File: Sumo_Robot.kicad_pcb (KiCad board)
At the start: 4 copper layers, 90 x 90 mm, 65 parts, among them J10 Screw_Terminal_01x03, J12 Screw_Terminal_01x02, J14 Screw_Terminal_01x02, J15 Conn_01x02, J16 Conn_01x03, J17 Conn_01x08, J18 Conn_01x02, J19 Conn_01x02, J2 Screw_Terminal_01x04, J3 Screw_Terminal_01x04, J4 Screw_Terminal_01x04, J5 Screw_Terminal_01x04, J6 Screw_Terminal_01x04, J7 Screw_Terminal_01x03, J8 Screw_Terminal_01x03, J9 Screw_Terminal_01x03, SW1 SW_SPST, SW3 SW_Omron_B3FS, U5 AMS1117-3.3, U6 TSOP38233

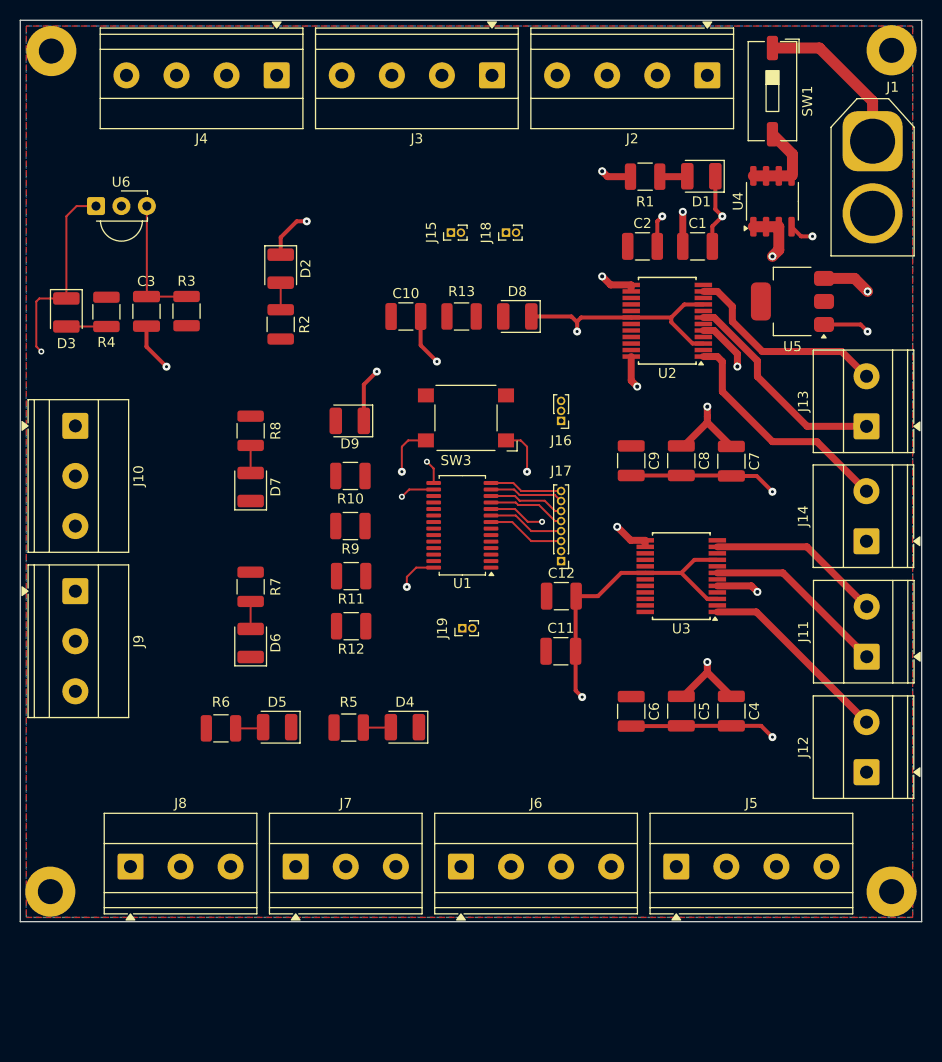
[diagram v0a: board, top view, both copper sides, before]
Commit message: updating layout
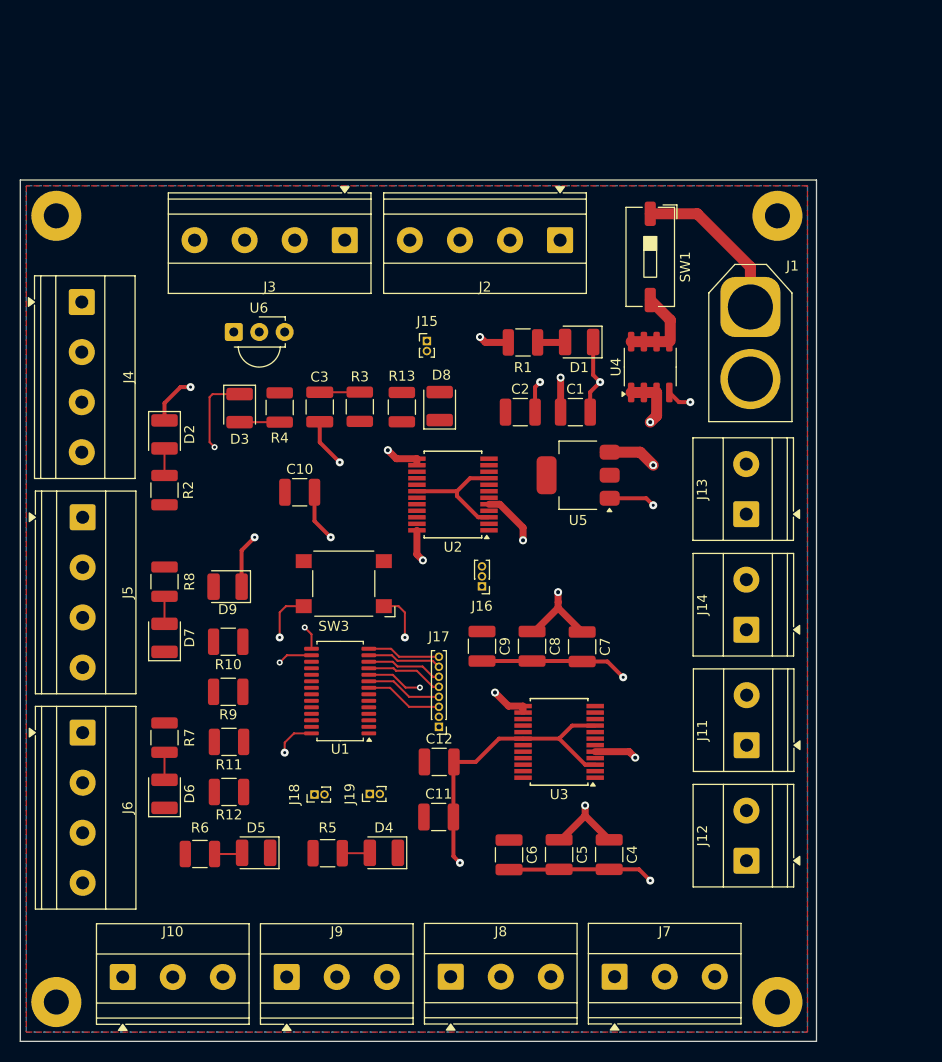
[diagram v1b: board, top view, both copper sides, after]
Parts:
- moved J5 68.8 mm to (110.1, 87.0), turned to -90 degrees
- moved J18 59.3 mm to (133.3, 114.7)
- moved J10 55.2 mm to (114.1, 133.0), turned to 0 degrees
- moved J9 43.9 mm to (130.5, 132.9), turned to 0 degrees
- moved J6 40.1 mm to (110.1, 108.5), turned to -90 degrees
- moved J8 33.8 mm to (146.9, 132.9)
- moved J7 33.7 mm to (163.2, 132.9)
- moved J4 29.8 mm to (110.0, 65.6), turned to -90 degrees
- moved U2 27.5 mm to (147.1, 84.8)
- moved U5 27.5 mm to (159.6, 82.8)
- moved C7 23.8 mm to (160.0, 100.0)
- moved C8 23.8 mm to (155.0, 99.9)
- moved C9 23.8 mm to (150.0, 99.9)
- moved J2 22.1 mm to (157.8, 59.4)
- moved J3 22.1 mm to (136.3, 59.4)
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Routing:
- net /InfraredReceiver/IR_RECEIVE: track 88.4 -> 14.0 mm
- net MR_A01: track 23.6 -> 0.00 mm
- net MR_A02: track 29.0 -> 5.64 mm
- net ML_A02: track 27.3 -> 4.25 mm
- net MR_B02: track 21.7 -> 0.00 mm
- net MR_B01: track 20.7 -> 0.00 mm
- net UNUSED_1: track 23.5 -> 3.48 mm
- net ML_A01: track 19.5 -> 0.00 mm
- net ML_B02: track 18.4 -> 0.00 mm
- net ML_B01: track 17.4 -> 0.00 mm
- net GND: track 137.4 -> 126.0 mm, vias 15 -> 14
- net Net-(U6-Vs): track 13.1 -> 4.06 mm
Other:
- board size 90 x 90 mm -> 79.5 x 86 mm
